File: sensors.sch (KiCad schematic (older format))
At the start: 11 parts

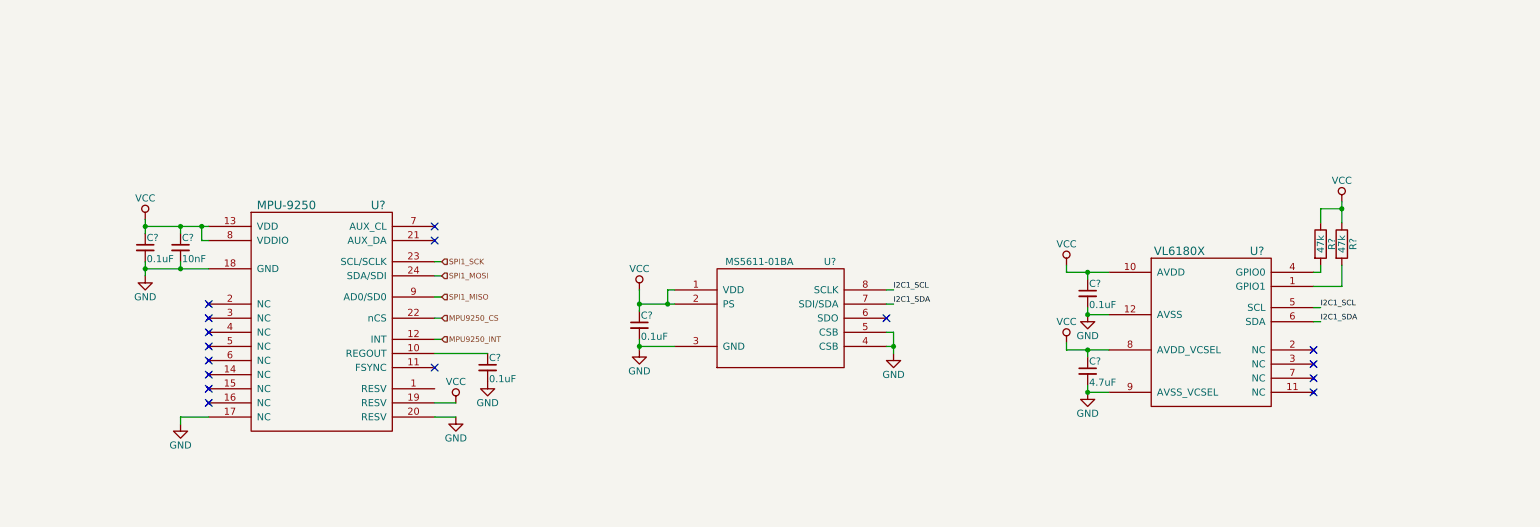
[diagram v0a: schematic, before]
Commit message: Annotation
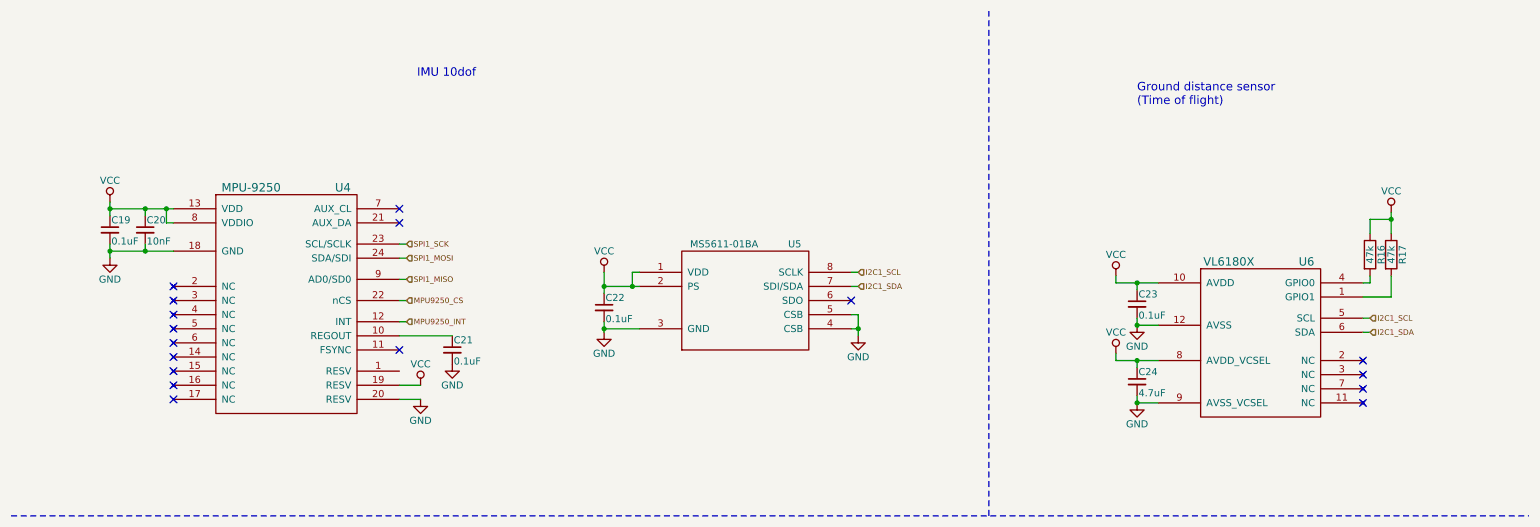
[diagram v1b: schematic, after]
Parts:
- gave numbers to parts that had none: 11
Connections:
- net GND: no longer U4.17 (NC)
- no-connect marks 16 -> 17
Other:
- note added: "Ground distance sensor \n(Time of flight)"
- note added: "IMU 10dof"
- moved on the sheet: C19, C20, C21, C22, C23, C24, R16, R17, U4, U5, U6
